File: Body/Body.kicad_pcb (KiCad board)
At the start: 2 copper layers, 127 x 100 mm, 30 parts, among them J1 Arduino_Nano_Header, J2 TB_1X2, J3 Cable_PAD, J4 TB_1X2, J5 TB_1X2, J6 Cable_PAD, J7 CONN_01X10, SW1 SW_SPDT, SW4 SW_Push, SW5 SW_Push, U1 DRV8833_MODULE, U2 LM78XX

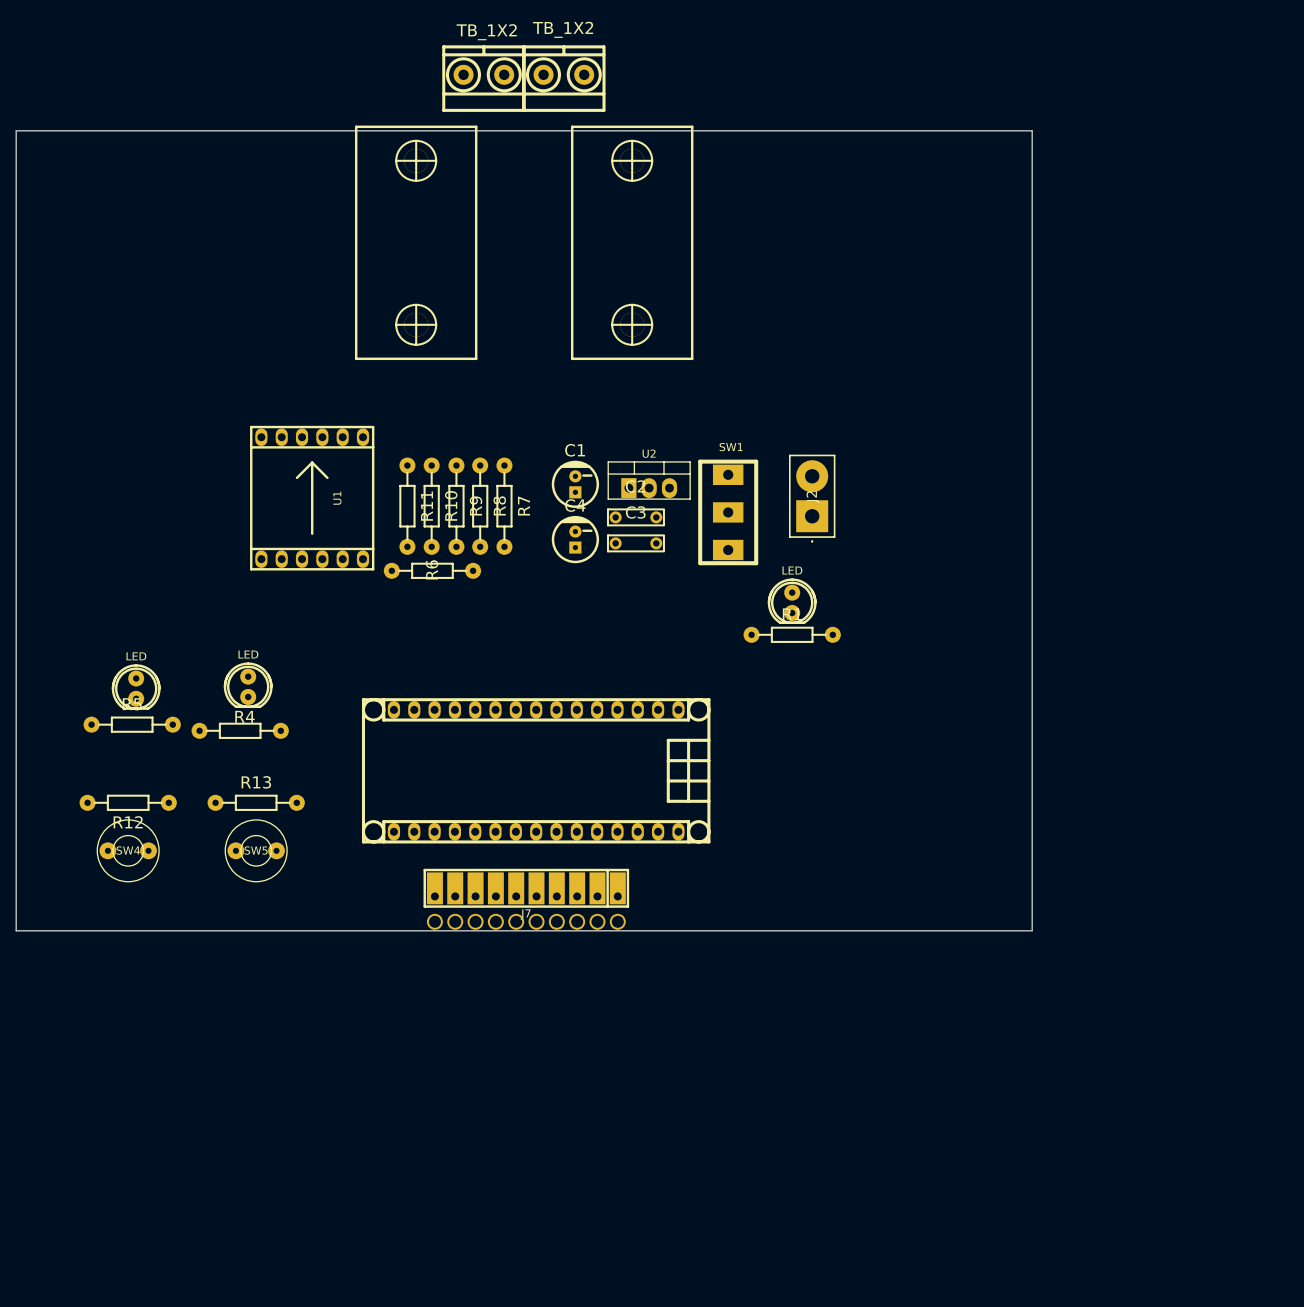
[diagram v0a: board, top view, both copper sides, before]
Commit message: rev_0.0.1
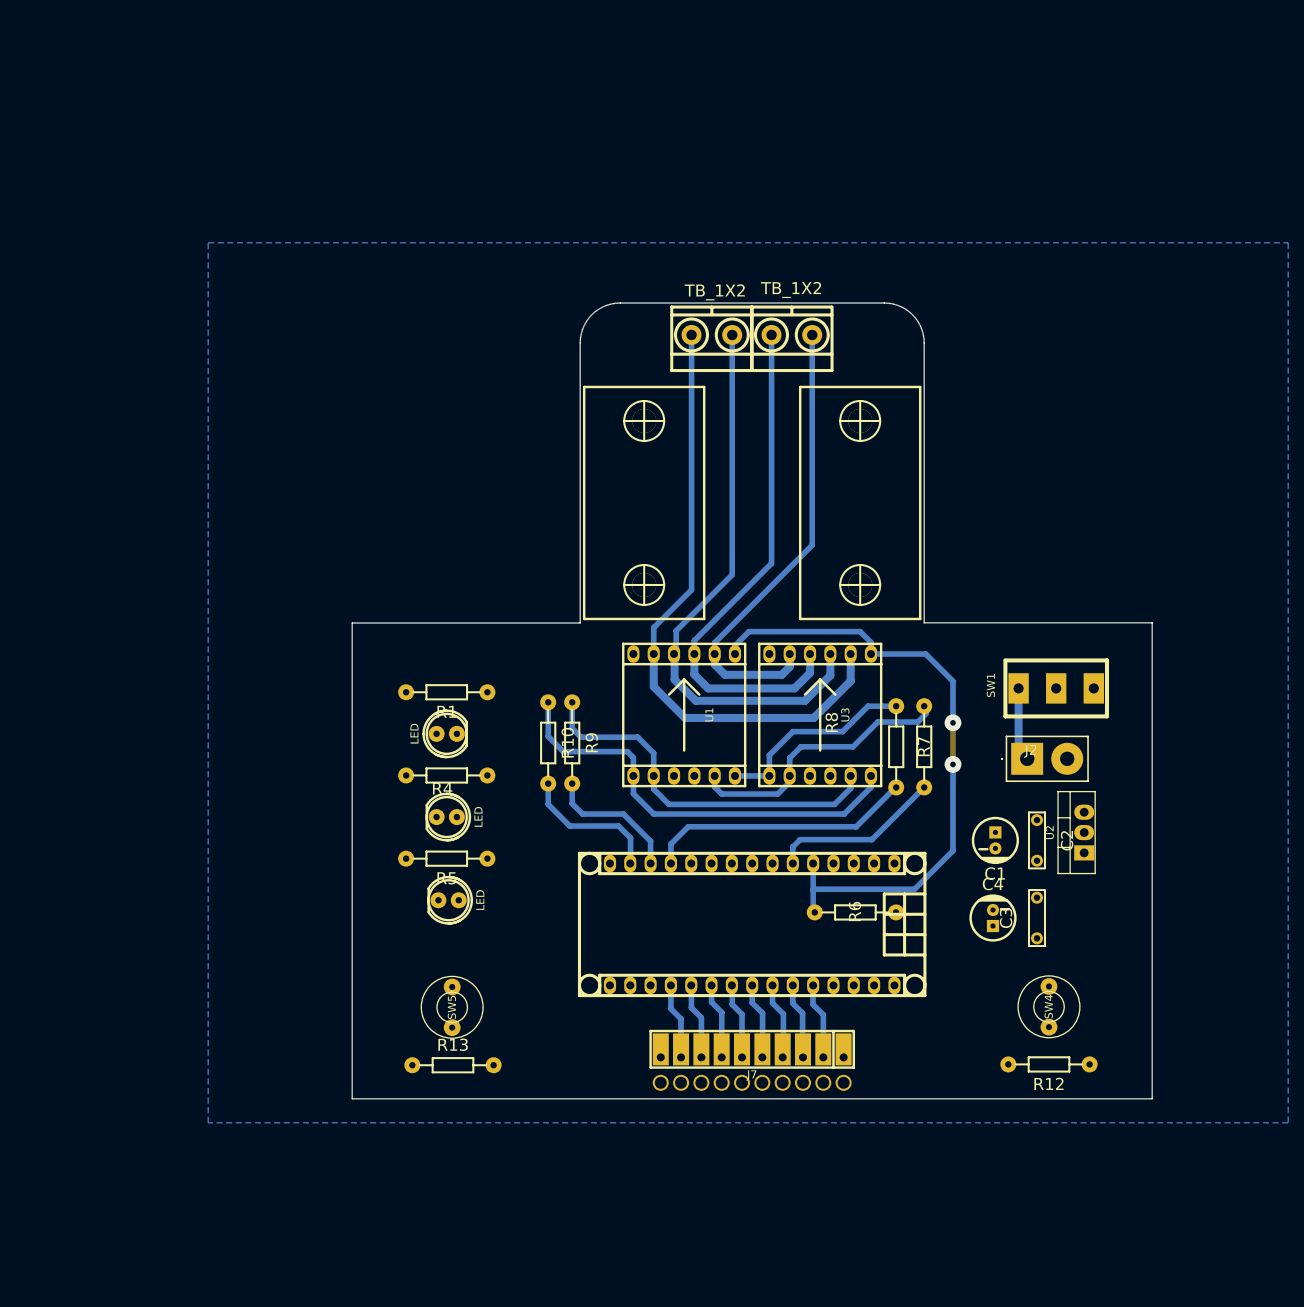
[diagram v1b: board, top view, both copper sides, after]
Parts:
- removed R11: R, MacroLib:RES0.3
- added U3: DRV8833_MODULE, MacroLib:DRV8833_MODULE, F.Cu at (146.5, 99.0)
- moved R12 119.7 mm to (175.1, 142.7)
- moved SW4 116.7 mm to (175.1, 135.5), turned to 90 degrees
- moved U2 72.9 mm to (179.5, 116.3), turned to 90 degrees
- moved C4 70.4 mm to (168.1, 124.4)
- moved C1 68.8 mm to (168.4, 114.7), turned to 180 degrees
- moved C3 68.6 mm to (173.6, 124.4), turned to 90 degrees
- moved R6 68.0 mm to (150.9, 123.7)
- moved C2 64.4 mm to (173.6, 114.7), turned to -90 degrees
- moved R7 60.5 mm to (159.5, 103.0)
- moved R8 60.1 mm to (156.0, 103.0), turned to 90 degrees
- moved U1 53.8 mm to (129.5, 99.0)
- moved LED3 47.2 mm to (100.0, 122.2), turned to -90 degrees
- moved SW1 46.5 mm to (176.0, 95.7), turned to 90 degrees
- moved LED1 46.2 mm to (99.8, 101.4), turned to 90 degrees
- moved J2 44.1 mm to (174.9, 104.5), turned to 0 degrees
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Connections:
- net Net-(U1-OUT1) renamed /OUT1
- net Net-(U1-OUT2) renamed /OUT2
- net Net-(U1-OUT3) renamed /OUT3
- net Net-(U1-OUT4) renamed /OUT4
- C1 pad 1: VCC -> +7.5V
- C2 pad 1: VCC -> +7.5V
- J1 pad 30: VCC -> +7.5V
- J1 pad 8: Net-(J1-D5/T1) -> unconnected-(J1-D5/T1-Pad8)
- J2 pad 1: Net-(SW1-A) -> VCC
- LED1 pad 1: VCC -> Net-(LED1-A)
- LED1 pad 2: Net-(LED1-K) -> GND
- R1 pad 1: Net-(LED1-K) -> +7.5V
- R1 pad 2: GND -> Net-(LED1-A)
- R7 pad 1: /IN1A -> /IN2A
- R8 pad 2: /IN2A -> /IN1A
- SW1 pad 1: Net-(SW1-A) -> VCC
- SW1 pad 2: VCC -> +7.5V
- U1 pad 12: /EN -> unconnected-(U1-EPP-Pad12)
- U2 pad 3: VCC -> +7.5V
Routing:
- net /ULT: track 0.00 -> 79.3 mm, vias 0 -> 2
- net /OUT1: track 0.00 -> 77.5 mm
- net /OUT2: track 0.00 -> 70.7 mm
- net /OUT3: track 0.00 -> 66.1 mm
- net /OUT4: track 0.00 -> 58.2 mm
- net /IN2B: track 0.00 -> 54.1 mm
- net /IN1B: track 0.00 -> 47.0 mm
- net /IN2A: track 0.00 -> 35.0 mm
- net Net-(J1-D9/0C1): track 0.00 -> 33.5 mm
- net /IN1A: track 0.00 -> 25.6 mm
- net Net-(J1-D3/INT1): track 0.00 -> 21.6 mm
- net Net-(J1-D11/MOSI): track 0.00 -> 17.8 mm
- net Net-(J1-D10/SS): track 0.00 -> 17.0 mm
- net /S5: track 0.00 -> 9.60 mm
- net /S4: track 0.00 -> 9.55 mm
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- added copper zone on B.Cu, net GND
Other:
- board size 127 x 100 mm -> 100 x 99.5 mm

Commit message: new
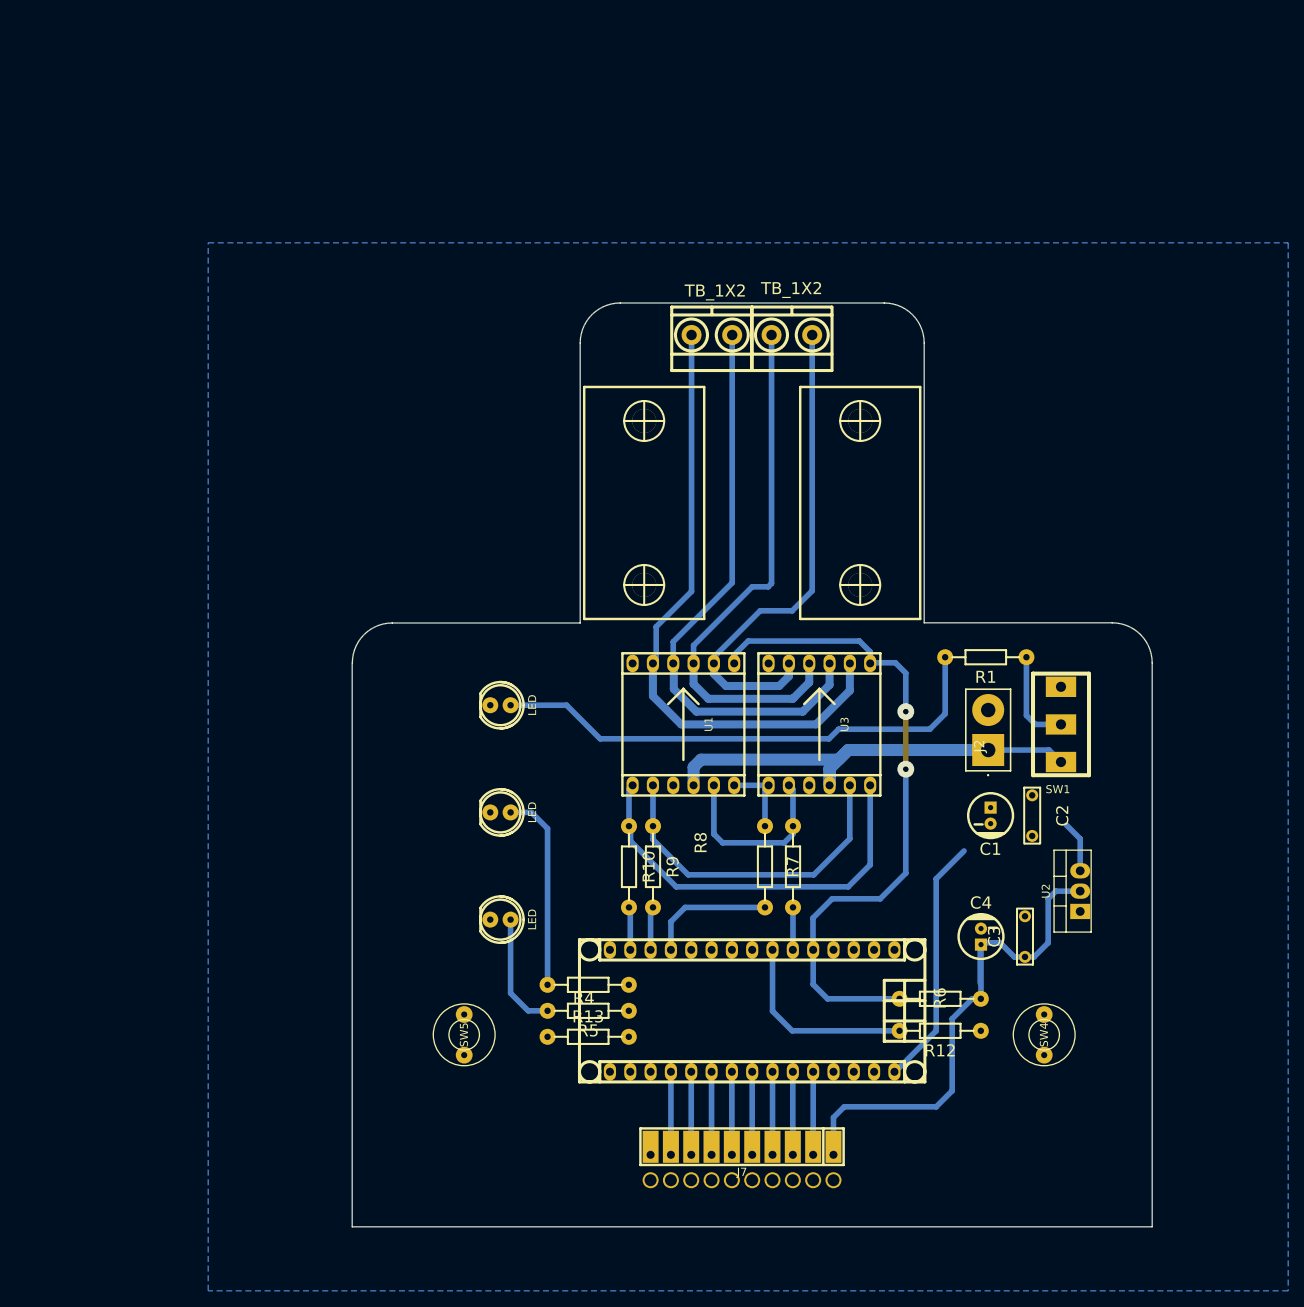
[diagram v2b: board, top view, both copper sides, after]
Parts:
- moved R1 67.5 mm to (167.2, 91.8)
- moved R4 31.6 mm to (117.5, 132.8)
- moved R5 26.0 mm to (117.5, 136.0)
- moved R7 22.2 mm to (143.1, 118.0)
- moved R8 22.2 mm to (139.6, 118.0)
- moved R10 18.5 mm to (122.6, 118.0)
- moved R9 18.5 mm to (125.6, 118.0)
- moved R13 17.3 mm to (117.5, 139.2)
- moved R6 15.1 mm to (161.5, 134.5)
- moved R12 14.2 mm to (161.5, 138.5)
- moved J7 12.2 mm to (136.7, 154.0)
- moved J1 10.8 mm to (138.0, 136.0)
- moved J2 8.24 mm to (167.5, 100.9), turned to 90 degrees
- moved LED1 7.61 mm to (106.5, 97.8), turned to -90 degrees
- moved U2 7.34 mm to (179.0, 123.6)
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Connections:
- J1 pad 10: /OUT_LED2 -> /OUT_LED1
- J1 pad 9: /OUT_LED1 -> /OUT_LED2
- LED2 pad 1: /OUT_LED1 -> Net-(LED2-A)
- LED2 pad 2: Net-(LED2-K) -> GND
- LED3 pad 1: /OUT_LED2 -> Net-(LED3-A)
- LED3 pad 2: Net-(LED3-K) -> GND
- R4 pad 1: Net-(LED2-K) -> /OUT_LED1
- R4 pad 2: GND -> Net-(LED2-A)
- R5 pad 1: Net-(LED3-K) -> /OUT_LED2
- R5 pad 2: GND -> Net-(LED3-A)
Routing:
- net +5V: track 0.00 -> 66.0 mm
- net Net-(LED1-A): track 0.00 -> 64.4 mm
- net +7.5V: track 0.00 -> 49.7 mm
- net VCC: track 9.25 -> 57.4 mm
- net /IN_BUTTON1: track 0.00 -> 25.1 mm
- net Net-(LED2-A): track 0.00 -> 25.0 mm
- net Net-(J1-D9/0C1): track 33.5 -> 16.0 mm
- net Net-(J1-D3/INT1): track 21.6 -> 5.31 mm
- net /IN1A: track 25.6 -> 9.59 mm
- net Net-(LED3-A): track 0.00 -> 14.7 mm
- net Net-(J1-D11/MOSI): track 17.8 -> 5.37 mm
- net /IN2A: track 35.0 -> 23.2 mm
- net Net-(J1-D10/SS): track 17.0 -> 5.43 mm
- net /IN1B: track 47.0 -> 41.8 mm
- net /ULT: track 79.3 -> 84.6 mm
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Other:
- board size 100 x 99.5 mm -> 100 x 115.5 mm
